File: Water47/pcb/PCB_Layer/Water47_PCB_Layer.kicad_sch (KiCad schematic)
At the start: 107 parts, among them SW1 Esc, SW10 O, SW11 P, SW12 -, SW13 Del, SW14 Cmd, SW15 A, SW16 S, SW17 D, SW18 F, SW19 G, SW2 Q, SW20 H, SW21 J, SW22 K, SW23 L, SW24 ;, SW25 Bs, SW26 Shift(L), SW27 Z, SW28 X, SW29 C, SW3 W, SW30 V, SW31 B, SW32 N, SW33 M, SW34 ,, SW35 ., SW36 Shift(R), SW37 Fn, SW38 Ctrl(L), SW39 Win(L), SW4 E, SW40 Alt(L), SW41 Shift(C), SW42 Fn(C), SW43 Enter, SW44 ←, SW45 ↓, SW46 ↑, SW47 →, SW5 R, SW6 T, SW7 Y, SW8 U, SW9 I, U1 MOUDLE-SEEEDUINO-XIAO

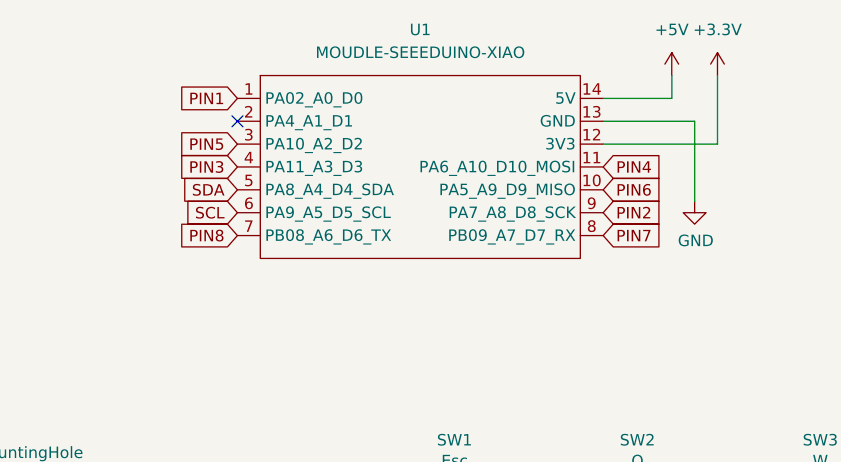
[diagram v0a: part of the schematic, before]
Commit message: feat: change micon direction
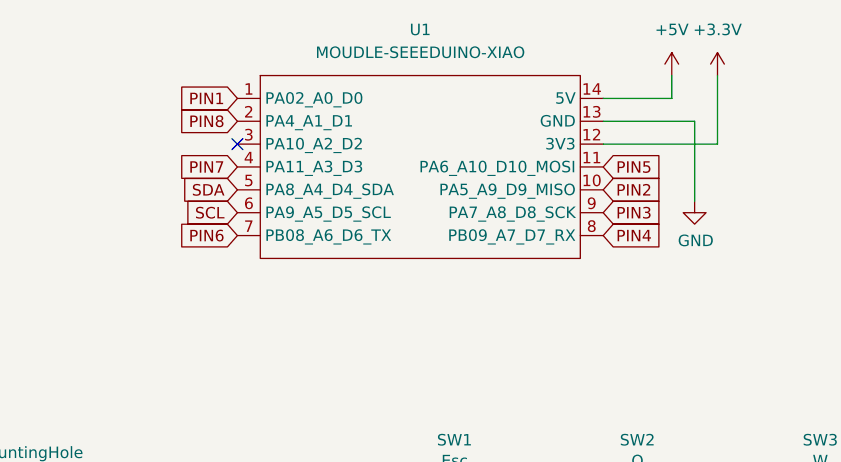
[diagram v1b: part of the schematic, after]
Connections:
- net PIN2: now also U1.10 (PA5_A9_D9_MISO); no longer U1.9 (PA7_A8_D8_SCK)
- net PIN3: now also U1.9 (PA7_A8_D8_SCK); no longer U1.4 (PA11_A3_D3)
- net PIN4: now also U1.8 (PB09_A7_D7_RX); no longer U1.11 (PA6_A10_D10_MOSI)
- net PIN5: now also U1.11 (PA6_A10_D10_MOSI); no longer U1.3 (PA10_A2_D2)
- net PIN6: now also U1.7 (PB08_A6_D6_TX); no longer U1.10 (PA5_A9_D9_MISO)
- net PIN7: now also U1.4 (PA11_A3_D3); no longer U1.8 (PB09_A7_D7_RX)
- net PIN8: now also U1.2 (PA4_A1_D1); no longer U1.7 (PB08_A6_D6_TX)
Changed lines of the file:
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@@
   (junction (at 71.12 163.83) (diameter 0) (color 0 0 0 0)
   )
-  (no_connect (at 54.61 33.02))
+  (no_connect (at 54.61 35.56))
   (wire (pts (xy 124.46 135.89) (xy 144.78 135.89))
     (stroke (width 0) (type default) (color 0 0 0 0))
@@
     )
   )
-  (global_label "PIN2" (shape input) (at 95.25 43.18 0) (fields_autoplaced)
+  (global_label "PIN1" (shape input) (at 54.61 30.48 180) (fields_autoplaced)
+    (effects (font (size 1.27 1.27)) (justify right))
+    (property "Intersheet References" "${INTERSHEET_REFS}" (id 0) (at 47.871 30.4006 0)
+      (effects (font (size 1.27 1.27)) (justify right) hide)
+    )
+  )
+  (global_label "PIN1" (shape input) (at 45.72 82.55 180) (fields_autoplaced)
+    (effects (font (size 1.27 1.27)) (justify right))
+    (property "Intersheet References" "${INTERSHEET_REFS}" (id 0) (at 38.981 82.4706 0)
+      (effects (font (size 1.27 1.27)) (justify right) hide)
+    )
+  )
+  (global_label "PIN7" (shape input) (at 54.61 38.1 180) (fields_autoplaced)
+    (effects (font (size 1.27 1.27)) (justify right))
+    (property "Intersheet References" "${INTERSHEET_REFS}" (id 0) (at 47.871 38.1794 0)
+      (effects (font (size 1.27 1.27)) (justify right) hide)
+    )
+  )
+  (global_label "PIN4" (shape input) (at 95.25 45.72 0) (fields_autoplaced)
     (effects (font (size 1.27 1.27)) (justify left))
-    (property "Intersheet References" "${INTERSHEET_REFS}" (id 0) (at 101.989 43.2594 0)
+    (property "Intersheet References" "${INTERSHEET_REFS}" (id 0) (at 101.989 45.6406 0)
       (effects (font (size 1.27 1.27)) (justify left) hide)
     )
   )
-  (global_label "PIN1" (shape input) (at 45.72 82.55 180) (fields_autoplaced)
-    (effects (font (size 1.27 1.27)) (justify right))
-    (property "Intersheet References" "${INTERSHEET_REFS}" (id 0) (at 38.981 82.4706 0)
-      (effects (font (size 1.27 1.27)) (justify right) hide)
-    )
-  )
-  (global_label "PIN4" (shape input) (at 95.25 38.1 0) (fields_autoplaced)
+  (global_label "PIN6" (shape input) (at 54.61 45.72 180) (fields_autoplaced)
+    (effects (font (size 1.27 1.27)) (justify right))
+    (property "Intersheet References" "${INTERSHEET_REFS}" (id 0) (at 47.871 45.6406 0)
+      (effects (font (size 1.27 1.27)) (justify right) hide)
+    )
+  )
+  (global_label "PIN5" (shape input) (at 95.25 38.1 0) (fields_autoplaced)
     (effects (font (size 1.27 1.27)) (justify left))
     (property "Intersheet References" "${INTERSHEET_REFS}" (id 0) (at 101.989 38.1794 0)
@@
     )
   )
-  (global_label "PIN6" (shape input) (at 95.25 40.64 0) (fields_autoplaced)
+  (global_label "PIN2" (shape input) (at 45.72 100.33 180) (fields_autoplaced)
+    (effects (font (size 1.27 1.27)) (justify right))
+    (property "Intersheet References" "${INTERSHEET_REFS}" (id 0) (at 38.981 100.2506 0)
+      (effects (font (size 1.27 1.27)) (justify right) hide)
+    )
+  )
+  (global_label "PIN5" (shape input) (at 45.72 153.67 180) (fields_autoplaced)
+    (effects (font (size 1.27 1.27)) (justify right))
+    (property "Intersheet References" "${INTERSHEET_REFS}" (id 0) (at 38.981 153.5906 0)
+      (effects (font (size 1.27 1.27)) (justify right) hide)
+    )
+  )
+  (global_label "PIN3" (shape input) (at 45.72 118.11 180) (fields_autoplaced)
+    (effects (font (size 1.27 1.27)) (justify right))
+    (property "Intersheet References" "${INTERSHEET_REFS}" (id 0) (at 38.981 118.0306 0)
+      (effects (font (size 1.27 1.27)) (justify right) hide)
+    )
+  )
+  (global_label "PIN7" (shape input) (at 45.72 189.23 180) (fields_autoplaced)
+    (effects (font (size 1.27 1.27)) (justify right))
+    (property "Intersheet References" "${INTERSHEET_REFS}" (id 0) (at 38.981 189.1506 0)
+      (effects (font (size 1.27 1.27)) (justify right) hide)
+    )
+  )
+  (global_label "PIN2" (shape input) (at 95.25 40.64 0) (fields_autoplaced)
     (effects (font (size 1.27 1.27)) (justify left))
-    (property "Intersheet References" "${INTERSHEET_REFS}" (id 0) (at 101.989 40.5606 0)
+    (property "Intersheet References" "${INTERSHEET_REFS}" (id 0) (at 101.989 40.7194 0)
       (effects (font (size 1.27 1.27)) (justify left) hide)
     )
   )
-  (global_label "PIN2" (shape input) (at 45.72 100.33 180) (fields_autoplaced)
-    (effects (font (size 1.27 1.27)) (justify right))
-    (property "Intersheet References" "${INTERSHEET_REFS}" (id 0) (at 38.981 100.2506 0)
-      (effects (font (size 1.27 1.27)) (justify right) hide)
-    )
-  )
-  (global_label "PIN7" (shape input) (at 95.25 45.72 0) (fields_autoplaced)
+  (global_label "SDA" (shape input) (at 54.61 40.64 180) (fields_autoplaced)
+    (effects (font (size 1.27 1.27)) (justify right))
+    (property "Intersheet References" "${INTERSHEET_REFS}" (id 0) (at 48.7177 40.5606 0)
+      (effects (font (size 1.27 1.27)) (justify right) hide)
+    )
+  )
+  (global_label "PIN6" (shape input) (at 45.72 171.45 180) (fields_autoplaced)
+    (effects (font (size 1.27 1.27)) (justify right))
+    (property "Intersheet References" "${INTERSHEET_REFS}" (id 0) (at 38.981 171.3706 0)
+      (effects (font (size 1.27 1.27)) (justify right) hide)
+    )
+  )
+  (global_label "PIN3" (shape input) (at 95.25 43.18 0) (fields_autoplaced)
     (effects (font (size 1.27 1.27)) (justify left))
-    (property "Intersheet References" "${INTERSHEET_REFS}" (id 0) (at 101.989 45.6406 0)
+    (property "Intersheet References" "${INTERSHEET_REFS}" (id 0) (at 101.989 43.1006 0)
       (effects (font (size 1.27 1.27)) (justify left) hide)
     )
   )
-  (global_label "PIN5" (shape input) (at 45.72 153.67 180) (fields_autoplaced)
-    (effects (font (size 1.27 1.27)) (justify right))
-    (property "Intersheet References" "${INTERSHEET_REFS}" (id 0) (at 38.981 153.5906 0)
-      (effects (font (size 1.27 1.27)) (justify right) hide)
-    )
-  )
-  (global_label "PIN3" (shape input) (at 45.72 118.11 180) (fields_autoplaced)
-    (effects (font (size 1.27 1.27)) (justify right))
-    (property "Intersheet References" "${INTERSHEET_REFS}" (id 0) (at 38.981 118.0306 0)
-      (effects (font (size 1.27 1.27)) (justify right) hide)
-    )
-  )
-  (global_label "PIN1" (shape input) (at 54.61 30.48 180) (fields_autoplaced)
-    (effects (font (size 1.27 1.27)) (justify right))
-    (property "Intersheet References" "${INTERSHEET_REFS}" (id 0) (at 47.871 30.4006 0)
-      (effects (font (size 1.27 1.27)) (justify right) hide)
-    )
-  )
-  (global_label "PIN7" (shape input) (at 45.72 189.23 180) (fields_autoplaced)
-    (effects (font (size 1.27 1.27)) (justify right))
-    (property "Intersheet References" "${INTERSHEET_REFS}" (id 0) (at 38.981 189.1506 0)
-      (effects (font (size 1.27 1.27)) (justify right) hide)
-    )
-  )
-  (global_label "PIN5" (shape input) (at 54.61 35.56 180) (fields_autoplaced)
-    (effects (font (size 1.27 1.27)) (justify right))
-    (property "Intersheet References" "${INTERSHEET_REFS}" (id 0) (at 47.871 35.4806 0)
-      (effects (font (size 1.27 1.27)) (justify right) hide)
-    )
-  )
-  (global_label "PIN3" (shape input) (at 54.61 38.1 180) (fields_autoplaced)
-    (effects (font (size 1.27 1.27)) (justify right))
-    (property "Intersheet References" "${INTERSHEET_REFS}" (id 0) (at 47.871 38.0206 0)
-      (effects (font (size 1.27 1.27)) (justify right) hide)
-    )
-  )
-  (global_label "SDA" (shape input) (at 54.61 40.64 180) (fields_autoplaced)
-    (effects (font (size 1.27 1.27)) (justify right))
-    (property "Intersheet References" "${INTERSHEET_REFS}" (id 0) (at 48.7177 40.5606 0)
-      (effects (font (size 1.27 1.27)) (justify right) hide)
-    )
-  )
-  (global_label "PIN6" (shape input) (at 45.72 171.45 180) (fields_autoplaced)
-    (effects (font (size 1.27 1.27)) (justify right))
-    (property "Intersheet References" "${INTERSHEET_REFS}" (id 0) (at 38.981 171.3706 0)
-      (effects (font (size 1.27 1.27)) (justify right) hide)
-    )
-  )
-  (global_label "PIN8" (shape input) (at 54.61 45.72 180) (fields_autoplaced)
-    (effects (font (size 1.27 1.27)) (justify right))
-    (property "Intersheet References" "${INTERSHEET_REFS}" (id 0) (at 47.871 45.7994 0)
-      (effects (font (size 1.27 1.27)) (justify right) hide)
-    )
-  )
   (global_label "PIN4" (shape input) (at 45.72 135.89 180) (fields_autoplaced)
     (effects (font (size 1.27 1.27)) (justify right))
@@
       (effects (font (size 1.27 1.27)) (justify right) hide)
     )
+  )
+  (global_label "PIN8" (shape input) (at 54.61 33.02 180) (fields_autoplaced)
+    (effects (font (size 1.27 1.27)) (justify right))
+    (property "Intersheet References" "${INTERSHEET_REFS}" (id 0) (at 47.871 33.0994 0)
+      (effects (font (size 1.27 1.27)) (justify right) hide)
+    )
